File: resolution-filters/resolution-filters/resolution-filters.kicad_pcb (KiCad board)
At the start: 2 copper layers, 91.7 x 48.8 mm, 52 parts, among them J501 Conn_Coaxial, J502 691137710002, J503 Conn_Coaxial, K501 G5V-1, K502 G5V-1, T501 Transformer_1P_1S, T502 Transformer_1P_1S, Y501 Crystal_GND3_Small, Y502 Crystal_GND3_Small, Y503 Crystal_GND3_Small, Y504 Crystal_GND3_Small

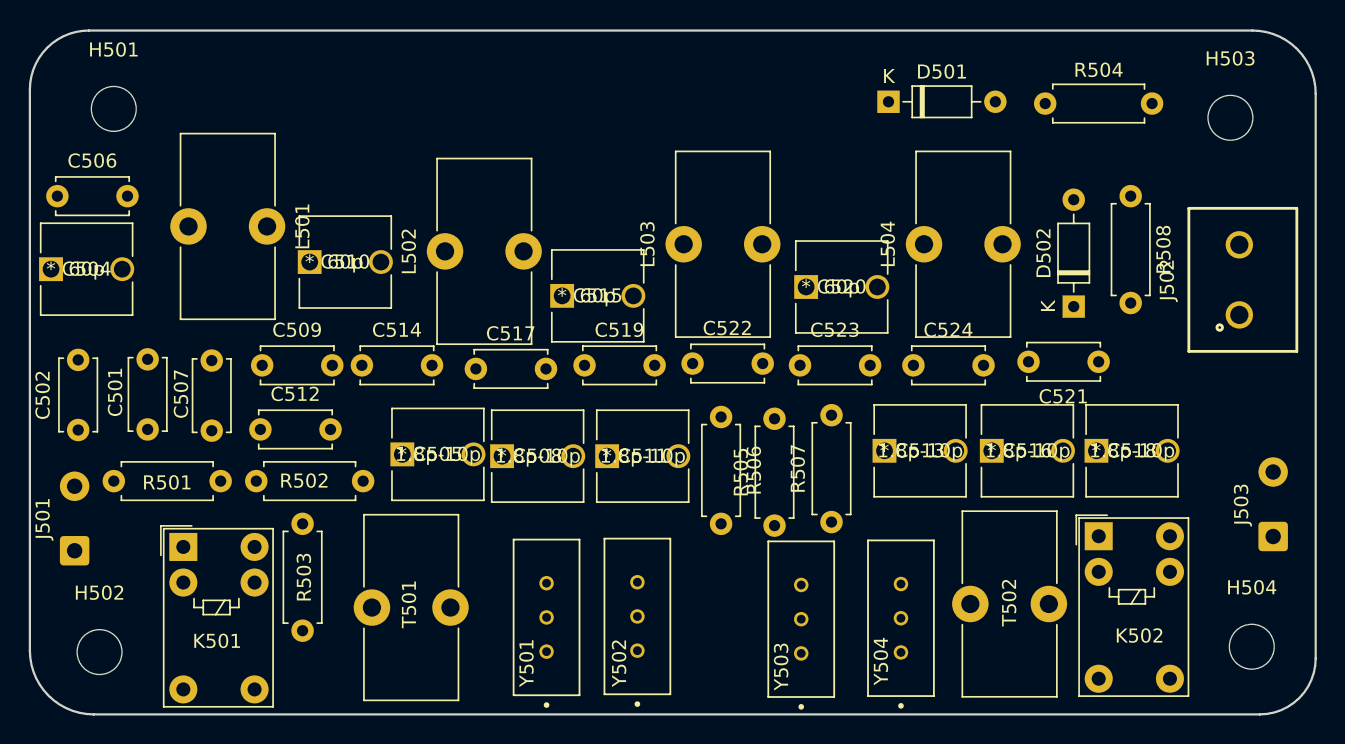
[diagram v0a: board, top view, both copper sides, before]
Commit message: resolution filter board layout
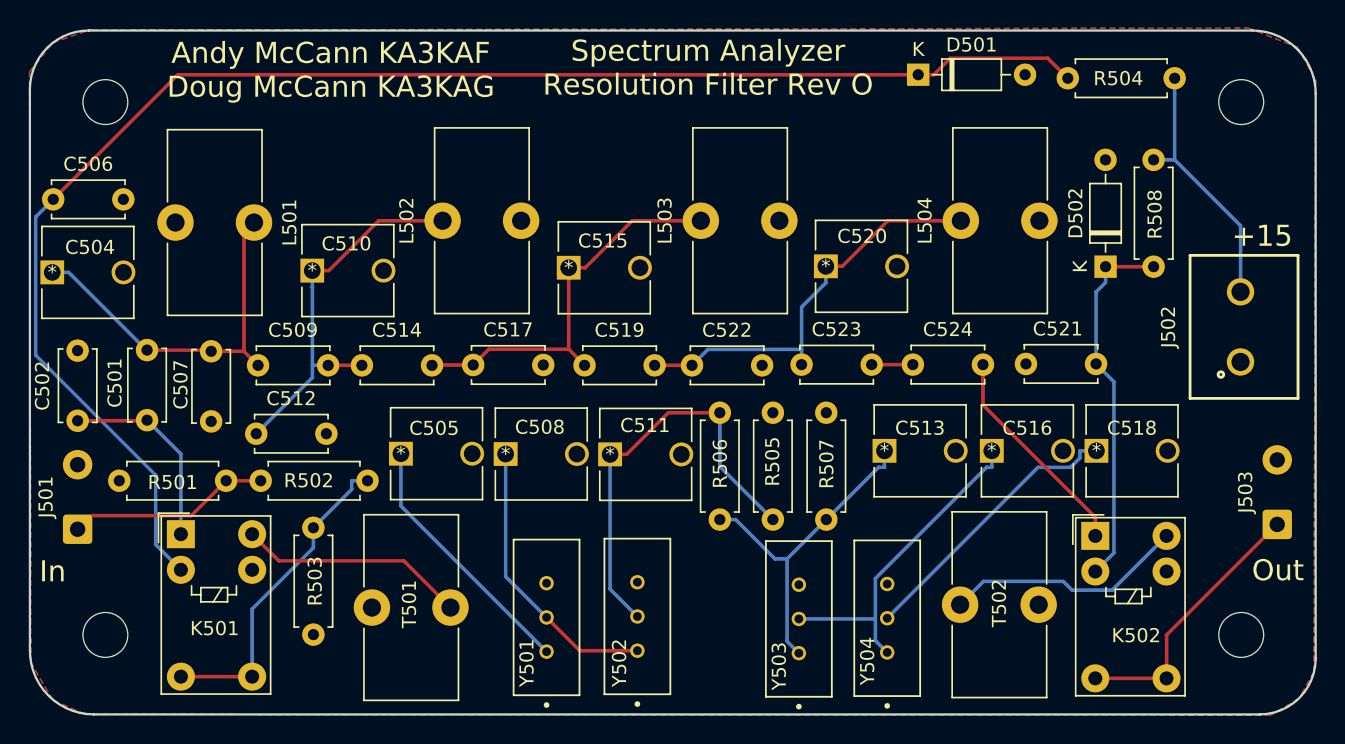
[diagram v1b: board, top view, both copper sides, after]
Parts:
- moved D502 3.64 mm to (177.8, 80.2)
- moved J502 3.35 mm to (187.5, 84.5)
- moved L504 3.12 mm to (167.5, 77.0)
- moved R508 3.06 mm to (181.3, 72.6)
- moved D501 2.87 mm to (164.5, 66.5)
- moved R504 2.42 mm to (175.1, 66.8)
- moved L502 2.19 mm to (130.6, 77.0)
- moved L503 2.08 mm to (149.0, 77.0)
- moved C515 2.06 mm to (139.5, 80.3)
- moved C520 2.04 mm to (157.9, 80.2)
- moved J501 1.55 mm to (104.5, 99.0)
- moved H503 1.36 mm to (187.5, 68.5)
- moved H502 1.29 mm to (106.5, 106.5)
- moved H504 1.13 mm to (187.5, 106.5)
- moved Y504 0.98 mm to (162.3, 105.3)
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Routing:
- net /501-in: track 0.00 -> 108.3 mm
- net Net-(C511-Pad1): track 0.00 -> 30.6 mm
- net Net-(C519-Pad2): track 0.00 -> 29.6 mm
- net Net-(C514-Pad2): track 0.00 -> 28.5 mm
- net Net-(C509-Pad2): track 0.00 -> 27.6 mm
- net Net-(C501-Pad1): track 0.00 -> 26.9 mm
- net /502-in: track 0.00 -> 26.5 mm
- net Net-(C513-Pad1): track 0.00 -> 23.9 mm
- net Net-(C516-Pad1): track 0.00 -> 23.8 mm
- net Net-(K501-Pad5): track 0.00 -> 23.1 mm
- net Net-(C508-Pad1): track 0.00 -> 20.3 mm
- net Net-(C518-Pad1): track 0.00 -> 20.2 mm
- net Net-(J503-Pad1): track 0.00 -> 19.3 mm
- net Net-(C503-Pad3): track 0.00 -> 18.7 mm
- net Net-(C505-Pad1): track 0.00 -> 18.4 mm
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- added copper zone on B.Cu, net GND
- added copper zone on F.Cu, net GND
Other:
- board text added: "+15"
- board text added: "Andy McCann KA3KAF Doug McCann KA3KAG"
- board text added: "In"
- board text added: "Out"
- board text added: "Spectrum Analyzer Resolution Filter Rev O"
